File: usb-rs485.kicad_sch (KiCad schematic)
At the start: 12 parts

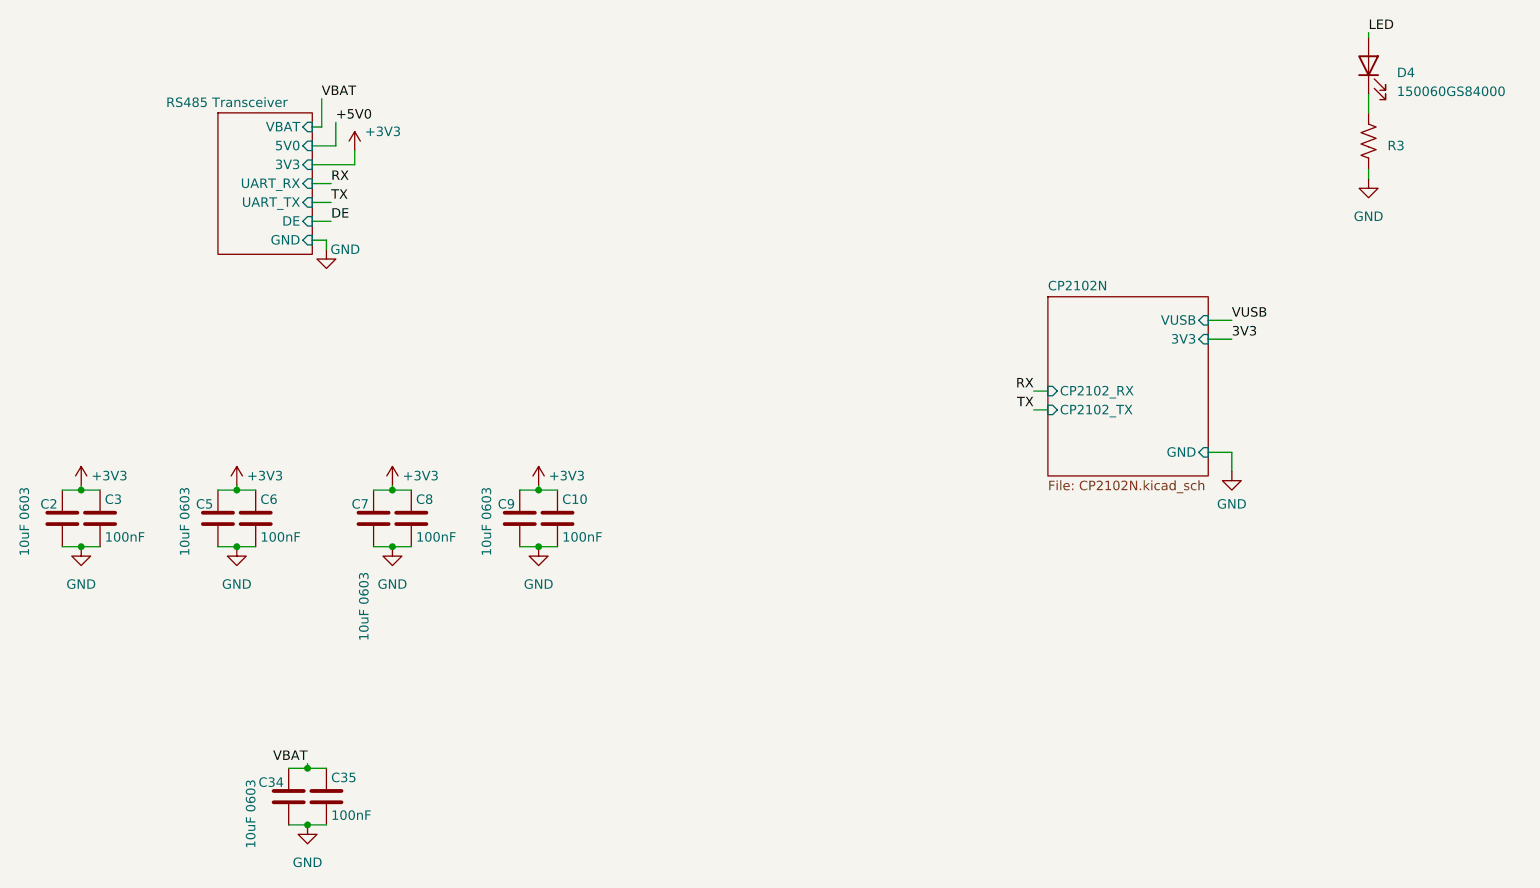
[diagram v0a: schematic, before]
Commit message: backups removalled schematic looking correct if not good
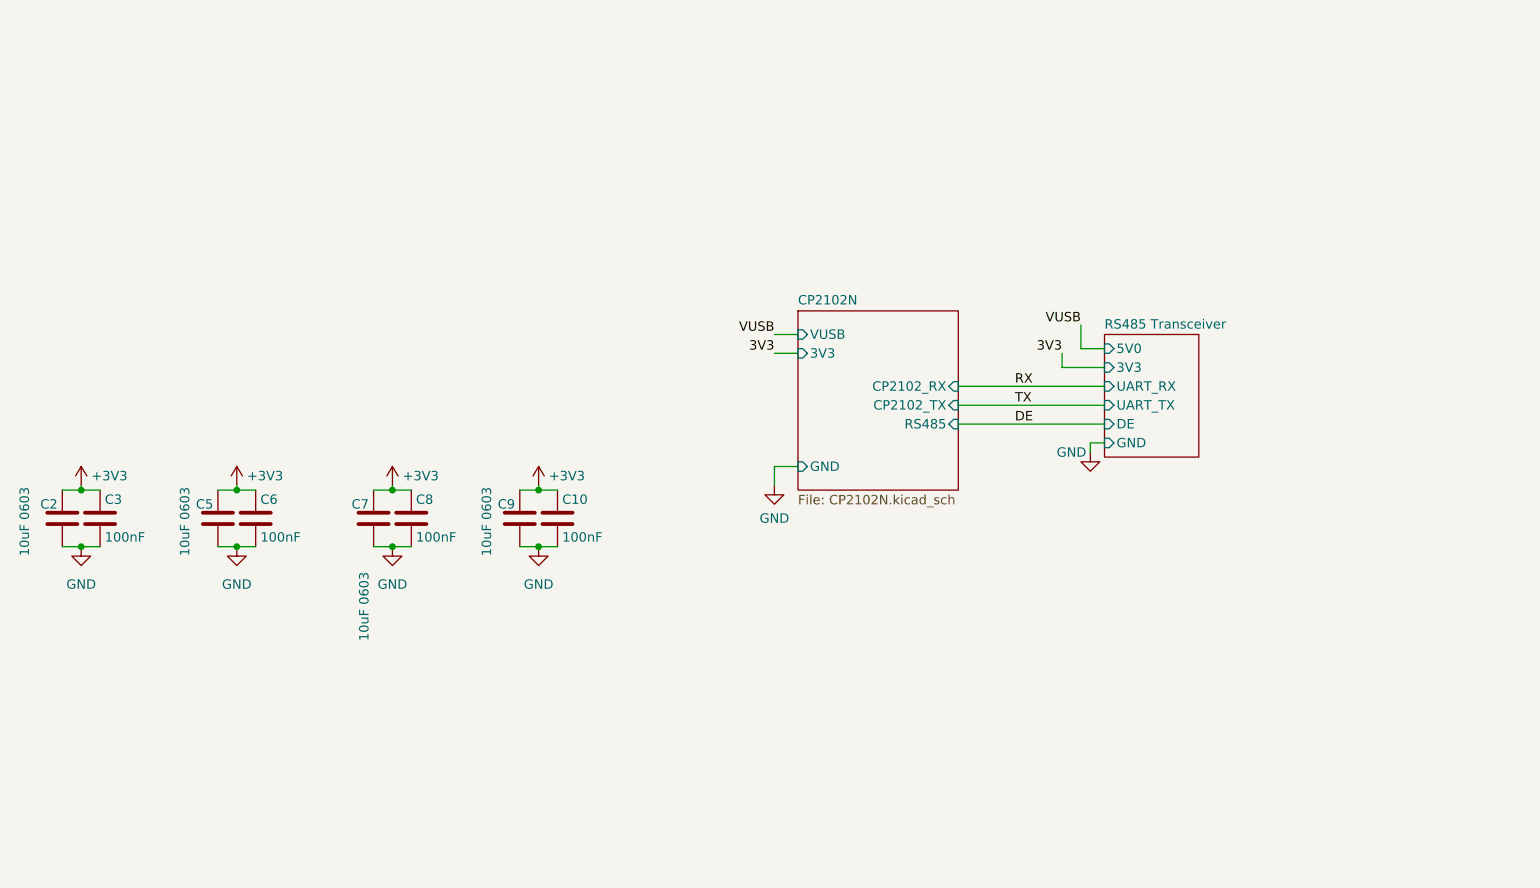
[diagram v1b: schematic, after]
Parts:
- removed C34: 10uF 0603, robot-cortex:C_0603_1608Metric, symbol foc-pcb:Capacitor
- removed C35: 100nF, robot-cortex:C_0402_1005Metric, symbol foc-pcb:Capacitor
- removed D4: 150060GS84000, robot-cortex:LED_0603_1608Metric, symbol foc-pcb:LED
- removed R3: 470, robot-cortex:R_0402_1005Metric, symbol foc-pcb:Resistor
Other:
- sheet CP2102N ports: added RS485; removed none
- sheet RS485 Transceiver ports: added none; removed VBAT
